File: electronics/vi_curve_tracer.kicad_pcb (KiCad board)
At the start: 2 copper layers, 27.9 x 38.1 mm, 29 parts, among them P1 CONN_01X05, P2 USB_OTG, P3 CONN_01X03, P4 CONN_01X03, U1 MCP6001, U2 pic24f08km202, U3 ft230x

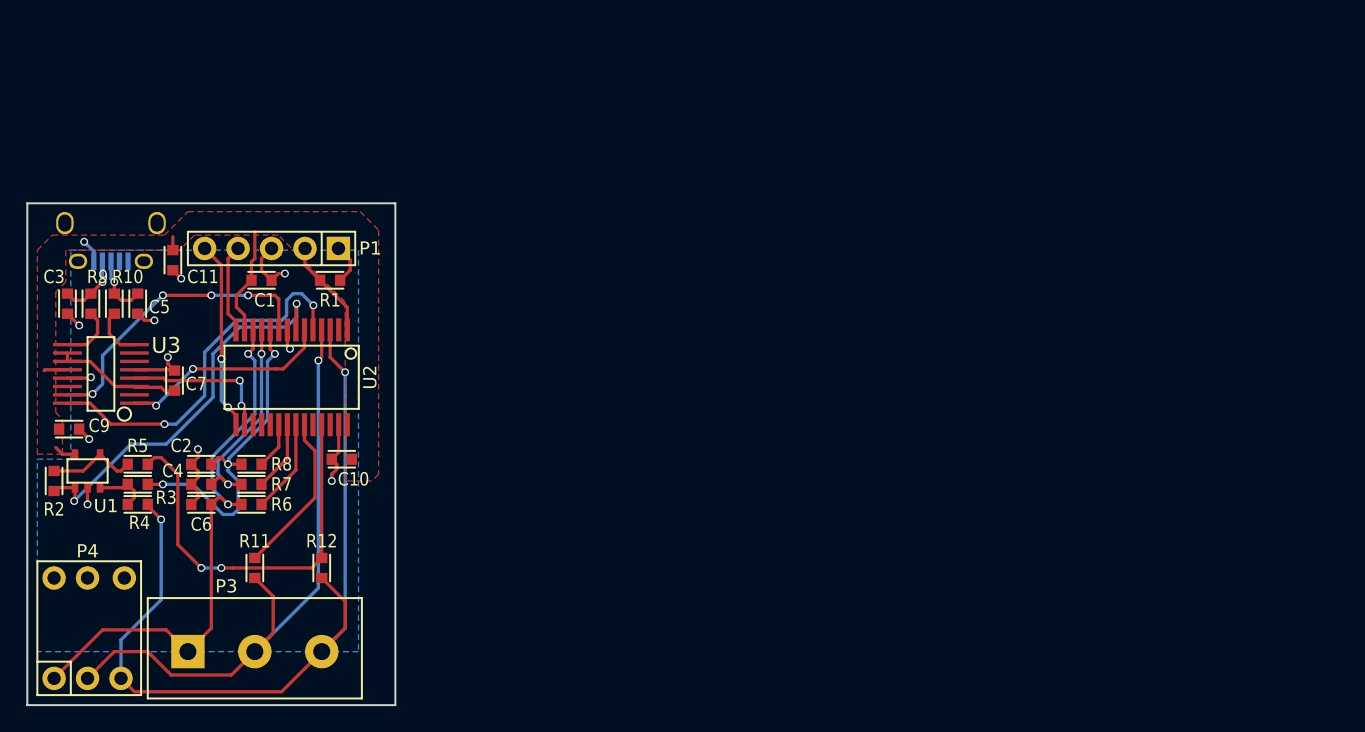
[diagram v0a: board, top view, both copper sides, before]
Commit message: Added electronics files, nearly complete
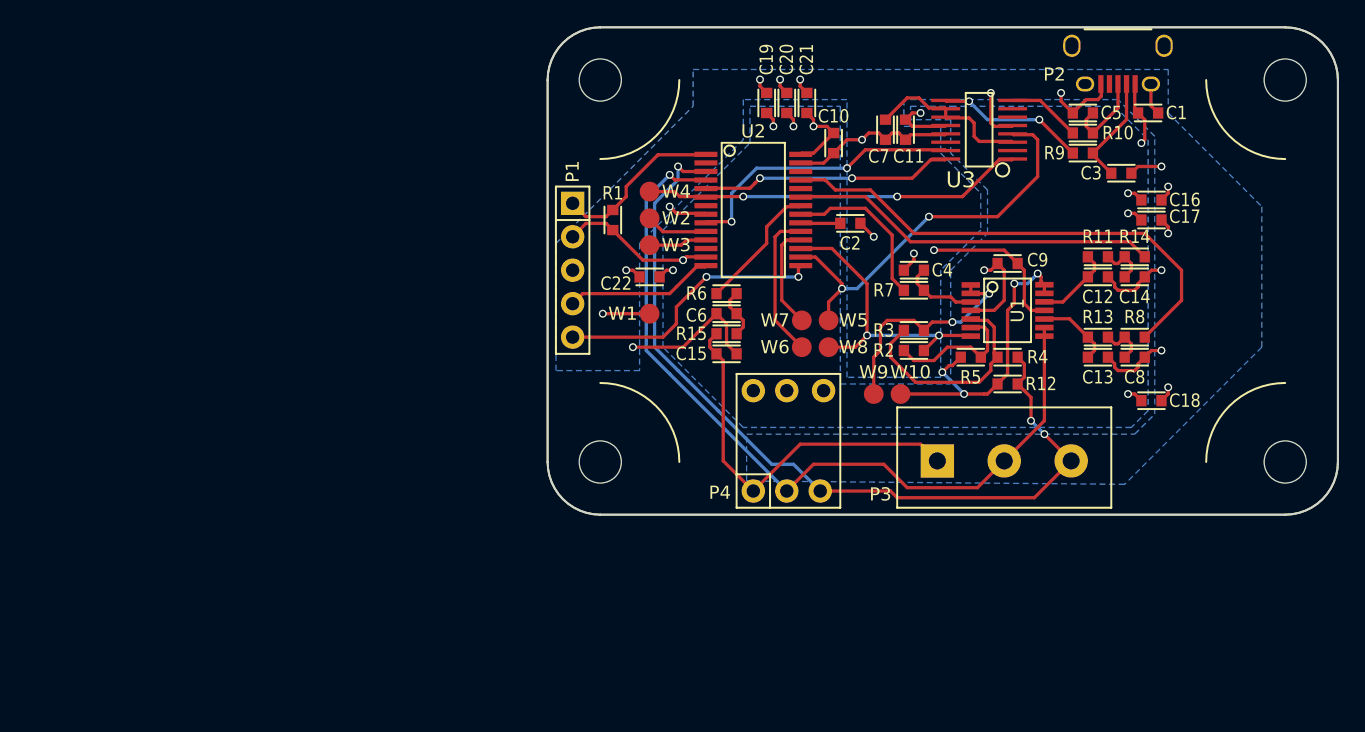
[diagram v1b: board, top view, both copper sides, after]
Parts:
- added C12: 100nF, kicad_pcb:SM_0603, F.Cu at (208.3, 91.9)
- added C13: 100nF, kicad_pcb:SM_0603, F.Cu at (208.3, 98.0)
- added C14: 100nF, kicad_pcb:SM_0603, F.Cu at (211.1, 91.9)
- added C15: 1uF, kicad_pcb:SM_0603, F.Cu at (180.1, 97.8)
- added C16: 1uF, kicad_pcb:SM_0603, F.Cu at (212.3, 86.1)
- added C17: 1uF, kicad_pcb:SM_0603, F.Cu at (212.3, 87.6)
- added C18: 1uF, kicad_pcb:SM_0603, F.Cu at (212.3, 101.3)
- added C19: 1uF, kicad_pcb:SM_0603, F.Cu at (183.1, 78.7)
- added C20: 1uF, kicad_pcb:SM_0603, F.Cu at (184.7, 78.7)
- added C21: 1uF, kicad_pcb:SM_0603, F.Cu at (186.2, 78.7)
- added C22: 1uF, kicad_pcb:SM_0603, F.Cu at (174.2, 91.9)
- added C8: 100nF, kicad_pcb:SM_0603, F.Cu at (211.1, 98.0)
- added R13: 1k, kicad_pcb:SM_0603, F.Cu at (208.3, 96.5)
- added R14: 1k, kicad_pcb:SM_0603, F.Cu at (211.1, 90.4)
- added R15: 1k, kicad_pcb:SM_0603, F.Cu at (180.1, 96.3)
- added REF**: case_sickOfBeige_60x37, kicad_pcb:case_sickOfBeige_60x37, F.Cu at (196.5, 91.5)
- added W1: TEST_1P, Measurement_Points:Measurement_Point_Round-SMD-Pad_Small, F.Cu at (174.2, 94.7)
- added W10: TEST_1P, Measurement_Points:Measurement_Point_Round-SMD-Pad_Small, F.Cu at (193.3, 100.8)
- added W2: TEST_1P, Measurement_Points:Measurement_Point_Round-SMD-Pad_Small, F.Cu at (174.2, 87.5)
- added W3: TEST_1P, Measurement_Points:Measurement_Point_Round-SMD-Pad_Small, F.Cu at (174.2, 89.5)
- added W4: TEST_1P, Measurement_Points:Measurement_Point_Round-SMD-Pad_Small, F.Cu at (174.2, 85.5)
- added W5: TEST_1P, Measurement_Points:Measurement_Point_Round-SMD-Pad_Small, F.Cu at (187.8, 95.2)
- added W6: TEST_1P, Measurement_Points:Measurement_Point_Round-SMD-Pad_Small, F.Cu at (185.8, 97.3)
- added W7: TEST_1P, Measurement_Points:Measurement_Point_Round-SMD-Pad_Small, F.Cu at (185.8, 95.2)
- added W8: TEST_1P, Measurement_Points:Measurement_Point_Round-SMD-Pad_Small, F.Cu at (187.8, 97.3)
- added W9: TEST_1P, Measurement_Points:Measurement_Point_Round-SMD-Pad_Small, F.Cu at (191.3, 100.8)
- P2: moved to F.Cu
- R12: value 100 -> 10
- R2, R3: value 10k -> 100k
- R6, R7, R8: value 100 -> 1k
- U1: value MCP6001 -> MCP6004; footprint kicad_pcb:SOT-23-5 -> SMD_Packages:SSOP-14
- moved C3 80.6 mm to (210.1, 84.1), turned to 0 degrees
- moved P2 77.6 mm to (209.8, 73.2), turned to 180 degrees
- moved R9 76.2 mm to (207.1, 82.5), turned to 0 degrees
- moved R10 74.7 mm to (207.1, 81.0), turned to 0 degrees
- moved C5 73.2 mm to (207.1, 79.5), turned to 180 degrees
- moved C9 72.3 mm to (201.4, 90.9)
- moved U1 70.9 mm to (201.4, 94.5), turned to 270 degrees
- moved U3 69.2 mm to (199.3, 80.8)
- moved C1 68.5 mm to (212.1, 79.5)
- moved R11 68.2 mm to (208.3, 90.4), turned to 0 degrees
- moved R8 67.7 mm to (211.1, 96.5)
- moved R4 67.0 mm to (201.4, 98.0)
- moved R2 66.0 mm to (194.3, 97.5), turned to 180 degrees
- moved R5 63.8 mm to (198.6, 98.0), turned to 0 degrees
- moved R3 60.1 mm to (194.3, 96.0)
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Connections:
- C2 pad 1: HZ_OUT_0 -> Net-(C2-Pad1)
- C4 pad 1: HZ_OUT_1 -> Net-(C4-Pad1)
- C6 pad 1: HZ_OUT_2 -> Net-(C6-Pad1)
- P1 pad 1: +5V -> ~MCLR
- P1 pad 2: ~MCLR -> +5V
- P3 pad 1: HZ_OUT_2 -> /GateVoltage
- P4 pad 1: HZ_OUT_2 -> /GateVoltage
- R11 pad 1: LD_VOLTAGE_0 -> Net-(C12-Pad1)
- R11 pad 2: LZ_OUT_0 -> Net-(C14-Pad1)
- R12 pad 1: LZ_OUT_1 -> /-Vout
- R3 pad 2: HZ_OUT_0 -> /IsenseReference
- R5 pad 1: LZ_OUT_1 -> /-Vout
- R6 pad 1: HZ_OUT_2 -> Net-(C6-Pad1)
- R7 pad 1: HZ_OUT_1 -> Net-(C4-Pad1)
- R8 pad 1: HZ_OUT_0 -> Net-(C8-Pad1)
- R8 pad 2: Net-(R8-Pad2) -> /DAC_high
- U1 pad 1: Net-(R2-Pad1) -> /IsenseReference
- U1 pad 2: GNDD -> /IsenseReference
- U1 pad 3: Net-(R3-Pad1) -> Net-(C4-Pad1)
- U1 pad 4: Net-(R2-Pad2) -> +5V
- U1 pad 5: +5V -> Net-(R3-Pad1)
- U2 pad 10: HZ_OUT_0 -> Net-(U2-Pad10)
- U2 pad 11: HZ_OUT_1 -> Net-(U2-Pad11)
- U2 pad 12: HZ_OUT_2 -> (no net)
- U2 pad 17: (no net) -> Net-(R2-Pad1)
- U2 pad 18: (no net) -> Net-(U2-Pad18)
- U2 pad 19: (no net) -> Net-(U2-Pad19)
- U2 pad 20: Net-(R8-Pad2) -> Net-(C2-Pad1)
- U2 pad 23: LZ_OUT_0 -> /DAC_low
- U2 pad 25: LZ_OUT_1 -> /DAC_high
- U2 pad 7: Net-(R2-Pad1) -> (no net)
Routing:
- net GNDD: track 27.9 -> 79.1 mm, vias 11 -> 19
- net HZ_OUT_2: track 42.5 -> 0.00 mm, vias 2 -> 0
- net /DAC_high: track 0.00 -> 38.0 mm
- net LZ_OUT_1: track 30.5 -> 0.00 mm, vias 2 -> 0
- net /GateVoltage: track 0.00 -> 29.5 mm
- net /DAC_low: track 0.00 -> 28.0 mm
- net HZ_OUT_0: track 26.2 -> 0.00 mm, vias 3 -> 0
- net /-Vout: track 0.00 -> 23.9 mm, vias 0 -> 4
- net +5V: track 18.1 -> 41.9 mm, vias 1 -> 11
- net FT230X_RX: track 11.6 -> 30.5 mm
- net /IsenseReference: track 0.00 -> 17.3 mm, vias 0 -> 2
- net HZ_OUT_1: track 16.1 -> 0.00 mm, vias 2 -> 0
- net LD_VOLTAGE_0: track 48.3 -> 62.4 mm
- net FT230X_TX: track 16.2 -> 28.9 mm
- net Net-(R3-Pad1): track 4.15 -> 16.9 mm
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- added copper zone on B.Cu, net +5V
- removed copper zone on F.Cu, net +5V
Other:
- board size 27.9 x 38.1 mm -> 60 x 37 mm
